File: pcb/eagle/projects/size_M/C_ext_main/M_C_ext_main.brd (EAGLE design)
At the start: 12 parts, among them U1 CP2104-F03-GM

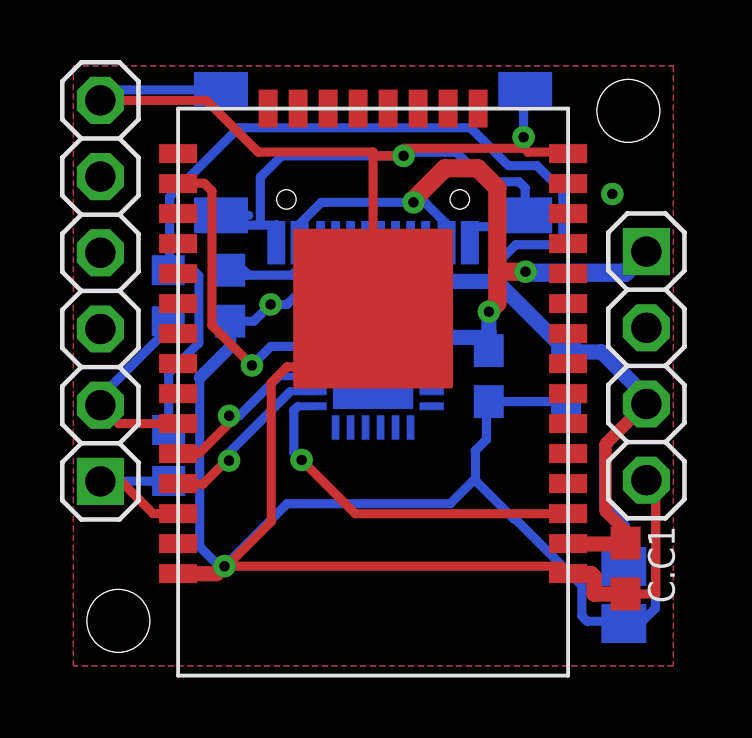
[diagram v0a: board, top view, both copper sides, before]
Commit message: PCB M.1
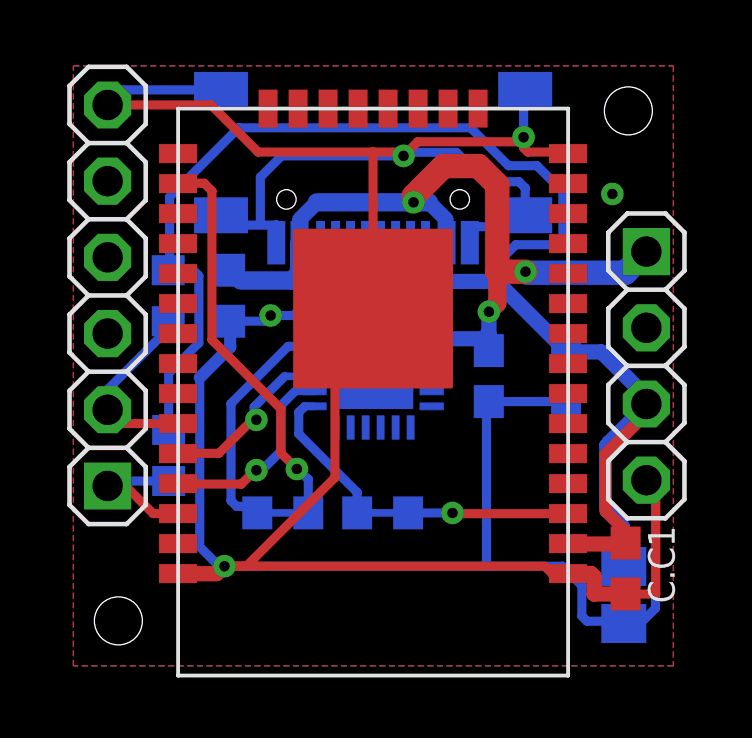
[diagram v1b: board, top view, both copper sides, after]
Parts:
- added C.R3, C.R4: 0, rcl:R0603
- moved C.J2 0.29 mm to (1.64, 12.8)
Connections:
- net PROG: now also C.R4.1, C.R4.2
- net RESET: now also C.R3.1, C.R3.2
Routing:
- net PROG: track 9.97 -> 22.9 mm
- net GND: track 130.4 -> 128.3 mm
- net RX: track 5.99 -> 6.92 mm
- net VUSB: track 29.3 -> 30.1 mm
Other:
- board text added: "main M.1"
- board text removed: "ESP M.1"

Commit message: updated PCBS after the version 1 delivery
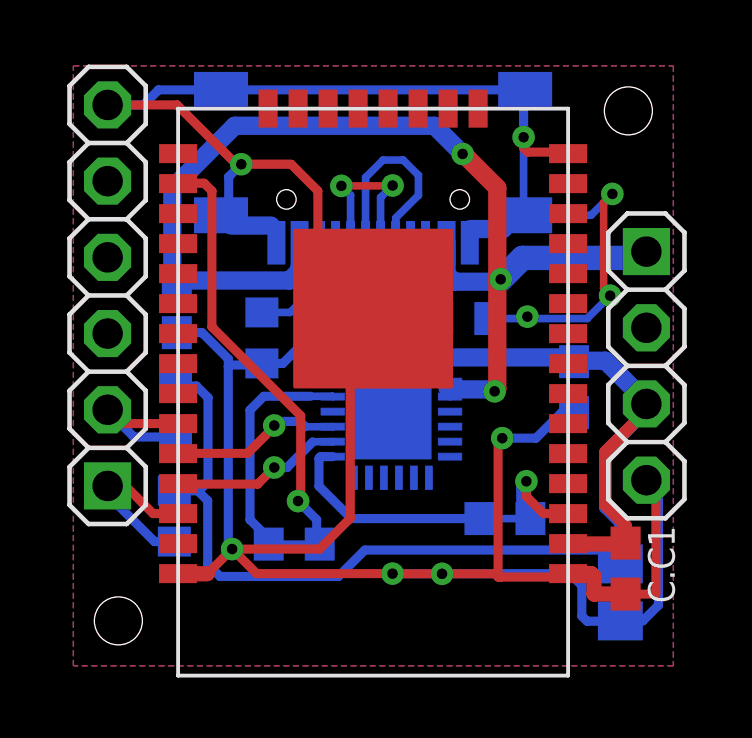
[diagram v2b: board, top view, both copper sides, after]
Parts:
- removed C.C4: 100n, rcl:C0603
- added C.R5: 5K1, rcl:R0603
- added C.R6: 5k1, rcl:R0603
- C.C5: value 10u -> 1u
- moved C.R3 4.08 mm to (14.9, 5.41)
- moved C.R2 3.87 mm to (3.90, 8.98)
- moved C.R1 2.03 mm to (3.87, 5.49)
- moved C.C5 1.82 mm to (3.95, 12.5)
- moved U1 1.78 mm to (11.1, 8.72)
- moved C.R4 1.11 mm to (7.86, 4.56)
- moved C.C2 0.44 mm to (17.2, 9.79)
- moved C.C3 0.14 mm to (18.7, 2.95)
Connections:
- removed net VIO: U1.5
- new net N$3: C.R6.2, U$1.A5
- new net N$4: C.R5.2, U$1.B5
- net GND: now also C.R5.1, C.R6.1; no longer C.C4.1
- net N$1: now also U$1.B7
- net N$2: now also U$1.B6
- net VCC: now also U1.5
- net VUSB: no longer C.C4.2
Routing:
- net N$2: track 2.25 -> 11.1 mm
- net VUSB: track 30.1 -> 38.7 mm
- net N$1: track 2.26 -> 9.99 mm, vias 0 -> 2
- net VCC: track 53.2 -> 46.2 mm
- net GND: track 128.3 -> 123.7 mm, vias 5 -> 9
- net N$3: track 0.00 -> 3.89 mm
- net N$4: track 0.00 -> 2.70 mm
- net SDA: track 6.33 -> 5.20 mm
- net RX: track 6.92 -> 5.81 mm
- net PROG: track 22.9 -> 24.0 mm
- net SCL: track 4.93 -> 5.89 mm
- net RESET: track 11.8 -> 12.7 mm
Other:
- board text added: "main M.2"
- board text removed: "main M.1"

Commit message: updated PCBs for version 2
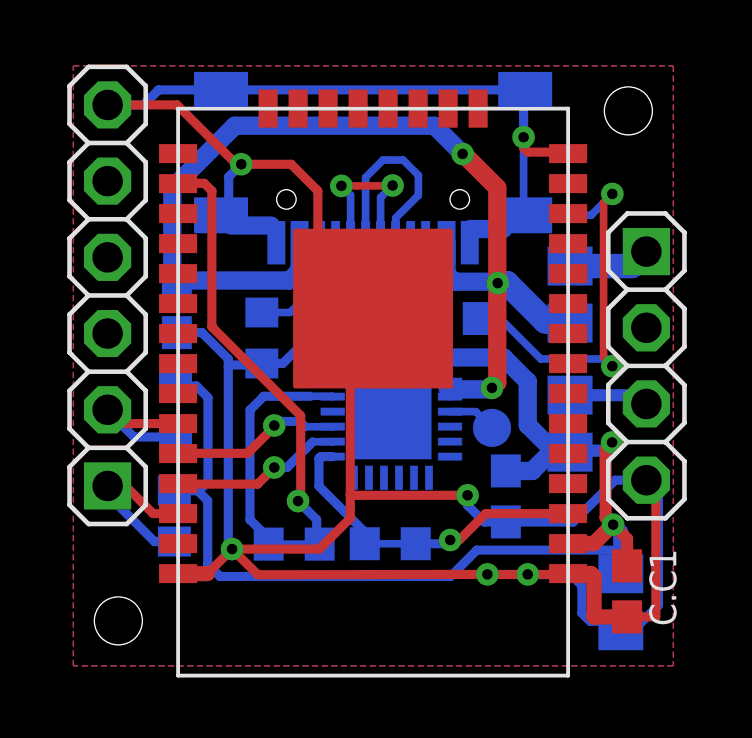
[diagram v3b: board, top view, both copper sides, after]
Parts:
- added C.F1, C.F2: (no value), rcl:R0805
- added PROGRAMMING: TPB1,27, testpad:B1,27
- moved C.C2 4.30 mm to (14.9, 6.15)
- moved C.R3 3.91 mm to (11.1, 4.57)
- moved C.C1 0.76 mm to (19.0, 2.98)
- moved C.R5 0.38 mm to (13.1, 12.1)
- moved C.C3 0.33 mm to (18.7, 2.62)
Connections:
- new net N$5: C.F2.2, JP1.3
- new net N$6: C.F1.2, JP1.1
- new net N$7: PROGRAMMING.TP, U1.9
- net VCC: now also C.F2.1; no longer JP1.3
- net VUSB: now also C.F1.1; no longer JP1.1
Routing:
- net GND: track 123.7 -> 128.9 mm, vias 9 -> 8
- net VCC: track 46.2 -> 43.4 mm, vias 0 -> 2
- net N$6: track 0.00 -> 2.74 mm
- net N$5: track 0.00 -> 2.67 mm
- net VUSB: track 38.7 -> 36.0 mm
- net N$7: track 0.00 -> 1.62 mm
- net RESET: track 12.7 -> 11.2 mm

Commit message: closed PCB version M.2
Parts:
- renumbered PROGRAMMING to PROG
